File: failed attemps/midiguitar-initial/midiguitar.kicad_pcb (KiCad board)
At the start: 2 copper layers, 72 x 32.9 mm, 13 parts, among them J1 PinHeader_01x06_P2.54mm_Verti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, J2 PinHeader_01x06_P2.54mm_Verti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, J3 NeoPixel, J4 Oled Display, M1 ESP32S3, SW1 Switch_Tactile_CUIDevices, U1 SN74LVC1T45DBVR

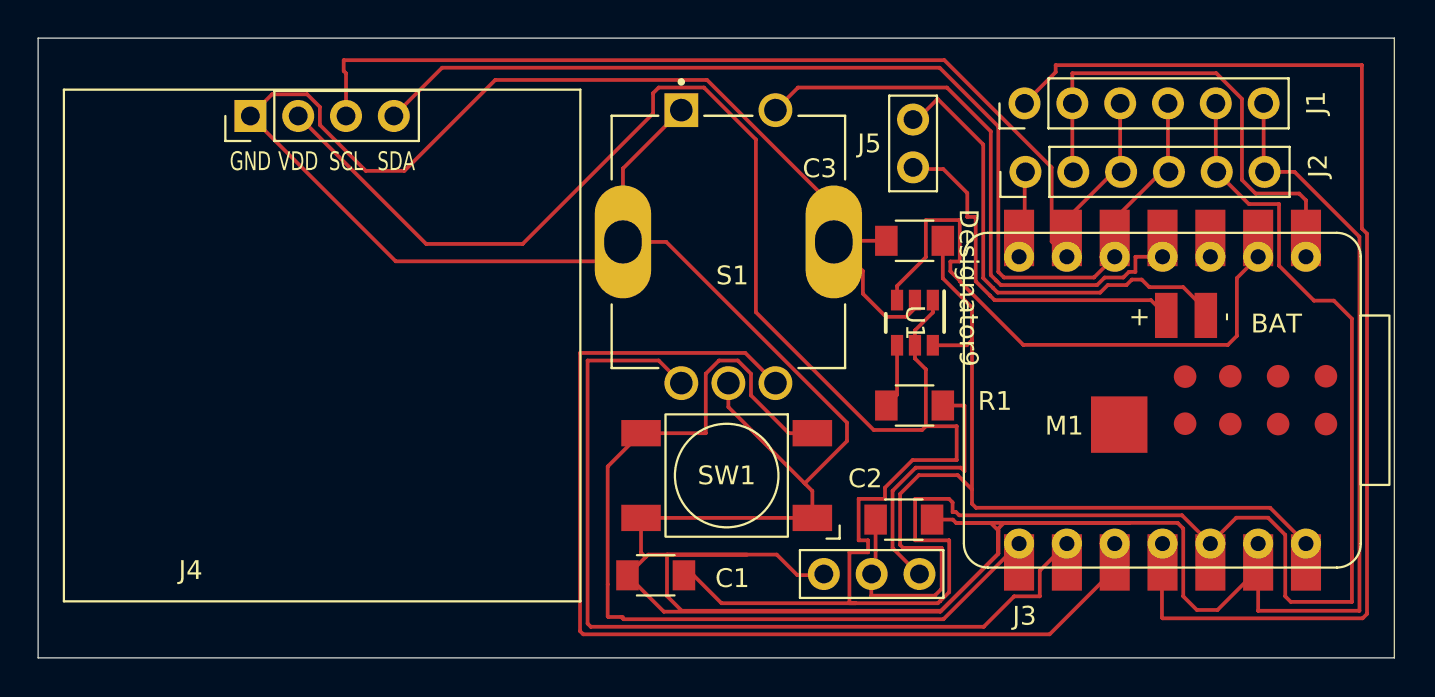
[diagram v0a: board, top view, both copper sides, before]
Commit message: Refactor code structure for improved readability and maintainability
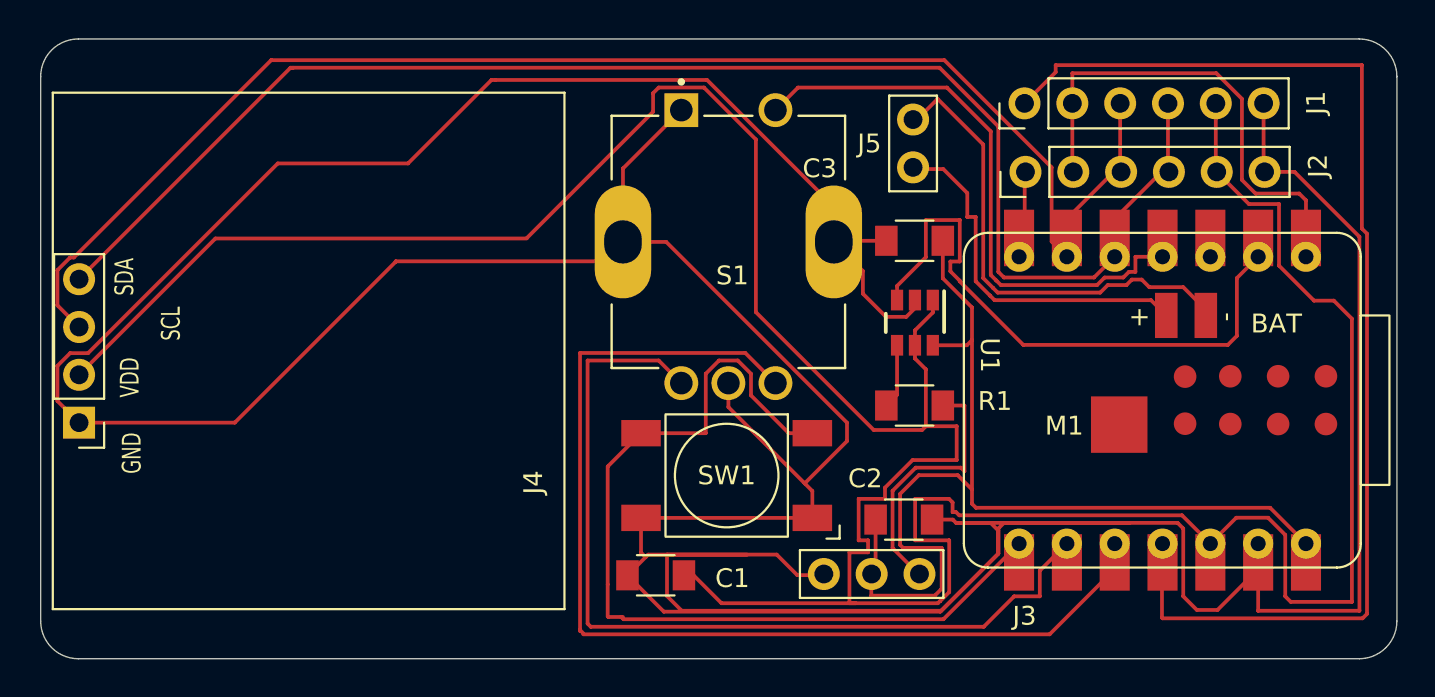
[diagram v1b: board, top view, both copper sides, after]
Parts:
- moved J4 18.0 mm to (117.3, 136.4), turned to 90 degrees
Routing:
- net PWR_GND: track 257.6 -> 282.4 mm
- net SDA: track 58.6 -> 79.0 mm
- net SCL: track 57.8 -> 78.1 mm
- net PWR_3V3: track 160.0 -> 171.6 mm
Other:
- outline, holes or cut-outs redrawn
